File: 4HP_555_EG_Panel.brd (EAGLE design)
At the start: 20.3 x 128.3 mm, 0 parts

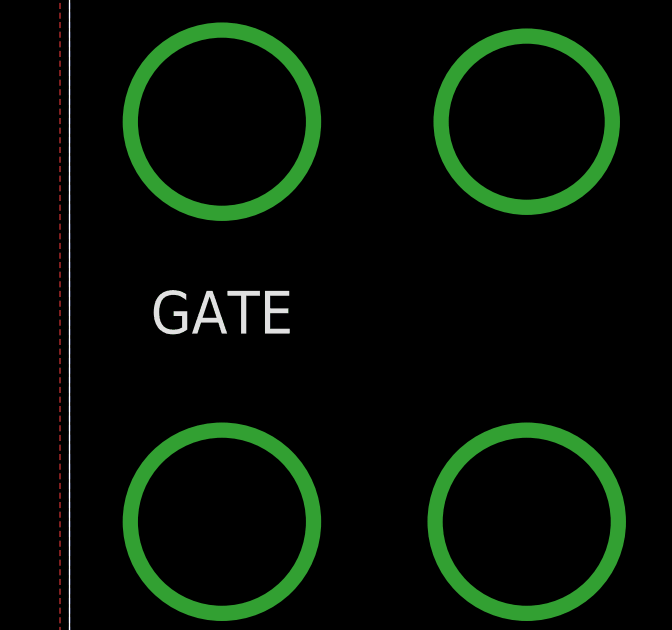
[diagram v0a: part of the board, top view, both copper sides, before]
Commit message: 4HP 555 ADSR EG
LM555 ADSR Envelope Generator
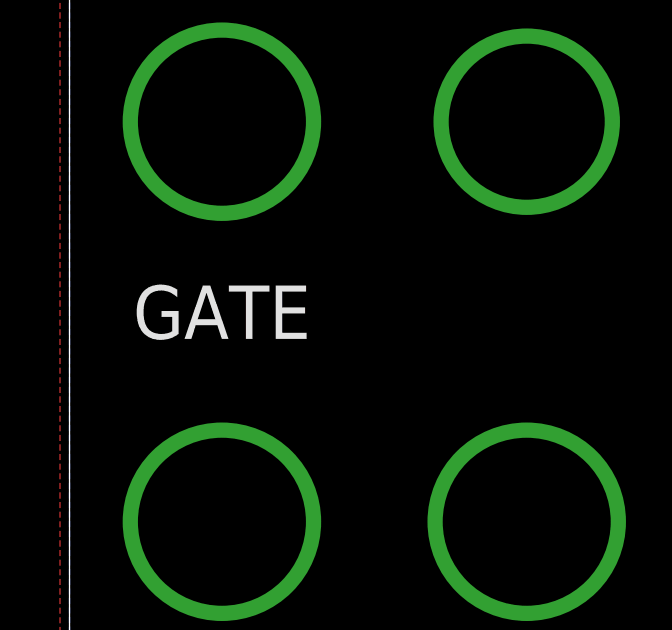
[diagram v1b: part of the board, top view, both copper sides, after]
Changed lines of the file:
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@@
 <?xml version="1.0" encoding="utf-8"?>
 <!DOCTYPE eagle SYSTEM "eagle.dtd">
-<eagle version="7.7.0">
+<eagle version="8.1.0">
 <drawing>
 <settings>
@@
 <text x="10.16" y="78.74" size="2.54" layer="21" font="vector" ratio="15" align="center">S</text>
 <text x="10.16" y="58.42" size="2.54" layer="21" font="vector" ratio="15" align="center">R</text>
-<text x="5.08" y="24.13" size="1.4224" layer="21" font="vector" ratio="15" align="center">GATE</text>
+<text x="5.08" y="24.13" size="1.778" layer="21" font="vector" ratio="15" align="center">GATE</text>
 <wire x1="13.335" y1="10.16" x2="14.605" y2="11.43" width="0.4064" layer="21"/>
 <wire x1="14.605" y1="11.43" x2="15.24" y2="10.795" width="0.4064" layer="21"/>
